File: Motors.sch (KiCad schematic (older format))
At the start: 5 parts

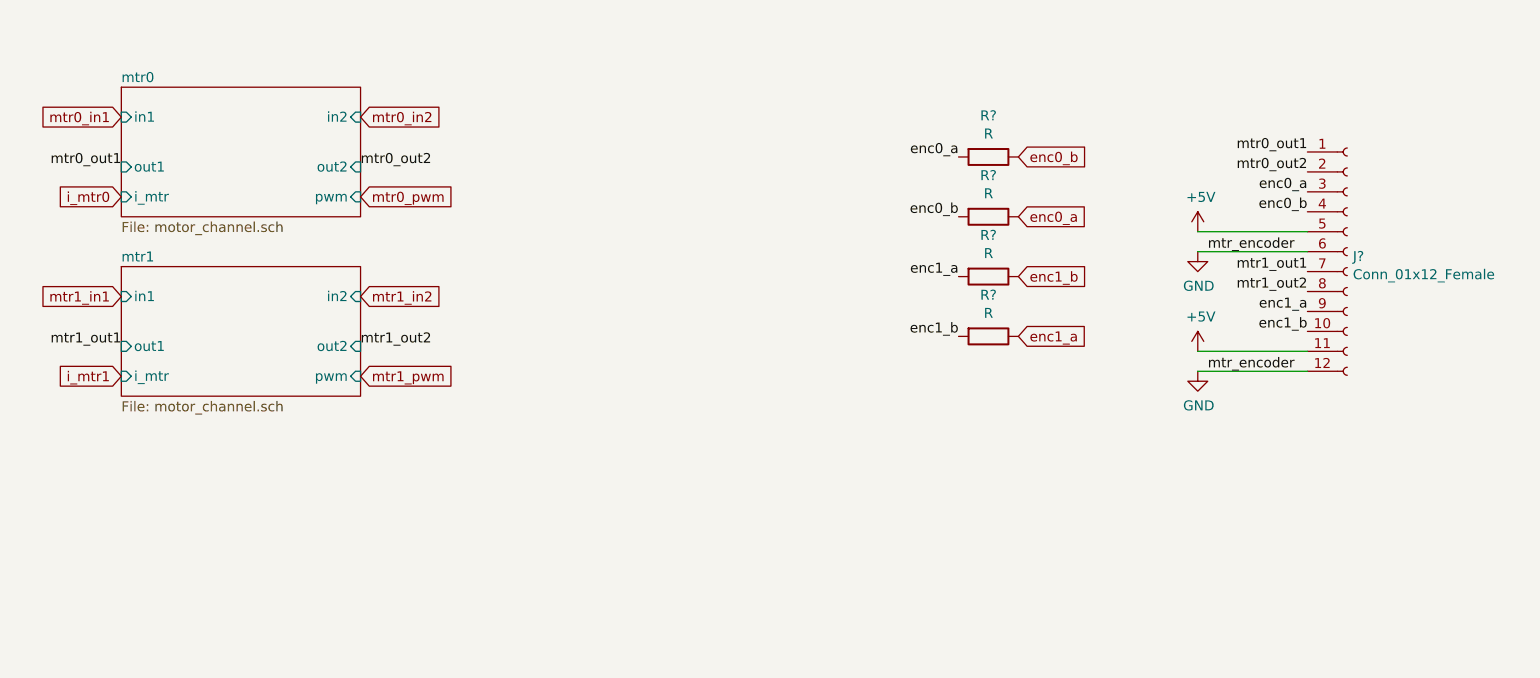
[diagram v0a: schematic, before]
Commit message: Motor capacitors, test points, jumpers
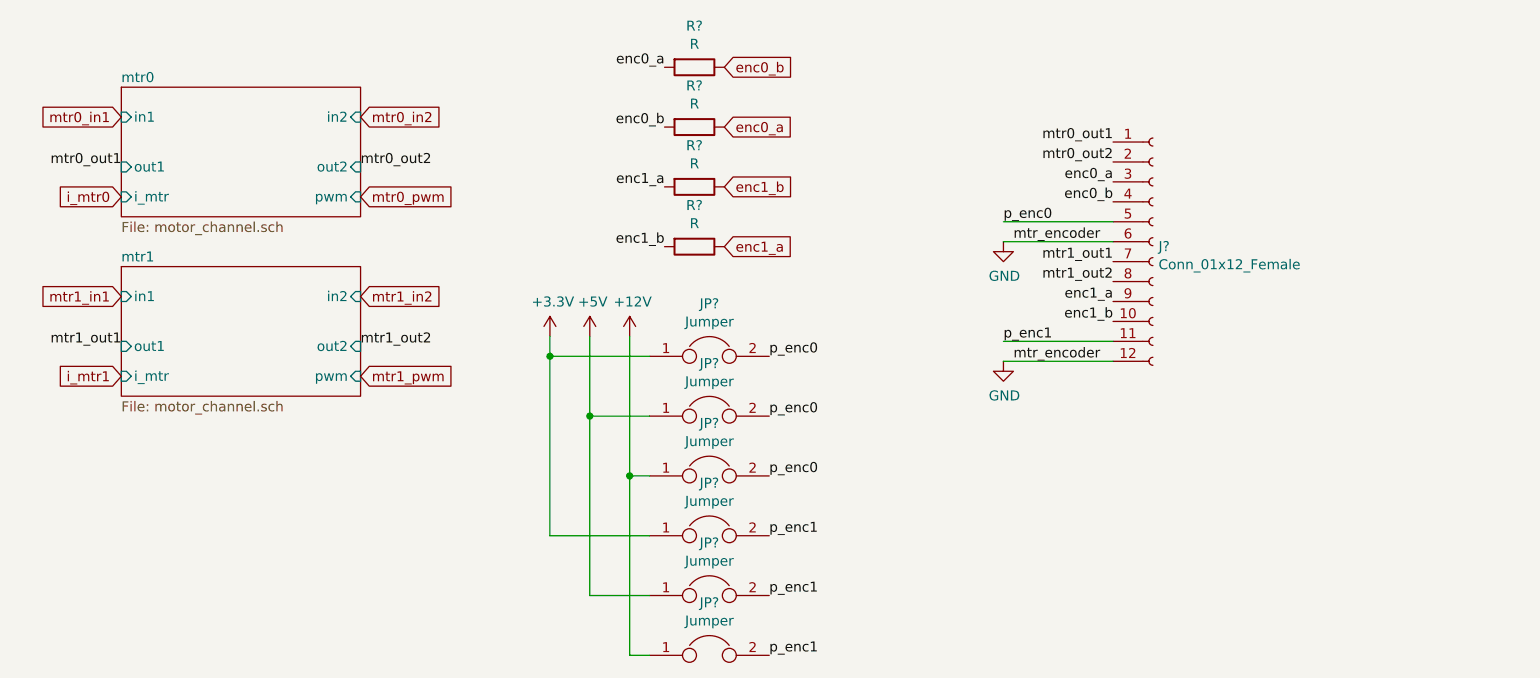
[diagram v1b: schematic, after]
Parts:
- added JP? (x6): Jumper, symbol Device:Jumper
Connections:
- net +5V: now also JP?.1, JP?.1; no longer J?.11 (Pin_11), J?.5 (Pin_5)
- new net +12V: JP?.1, JP?.1
- new net +3V3: JP?.1, JP?.1
- new net p_enc0: J?.5 (Pin_5), JP?.2, JP?.2, JP?.2
- new net p_enc1: J?.11 (Pin_11), JP?.2, JP?.2, JP?.2
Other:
- moved on the sheet: J?, R?
